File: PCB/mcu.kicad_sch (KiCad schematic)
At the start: 26 parts

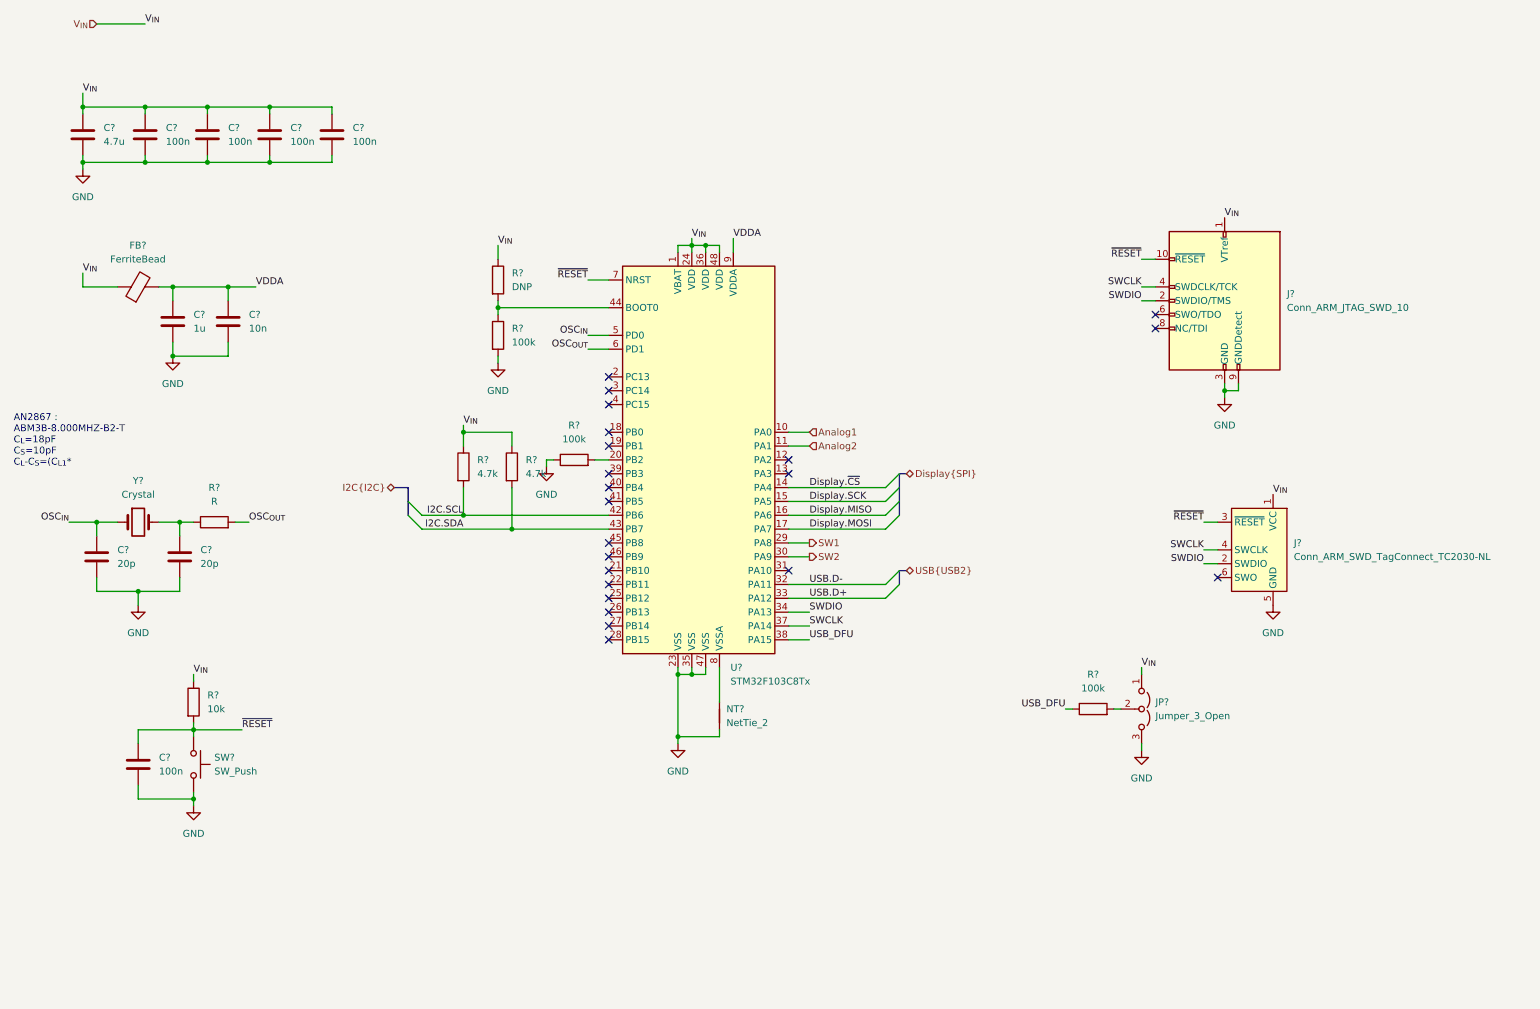
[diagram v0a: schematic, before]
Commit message: ok mcu
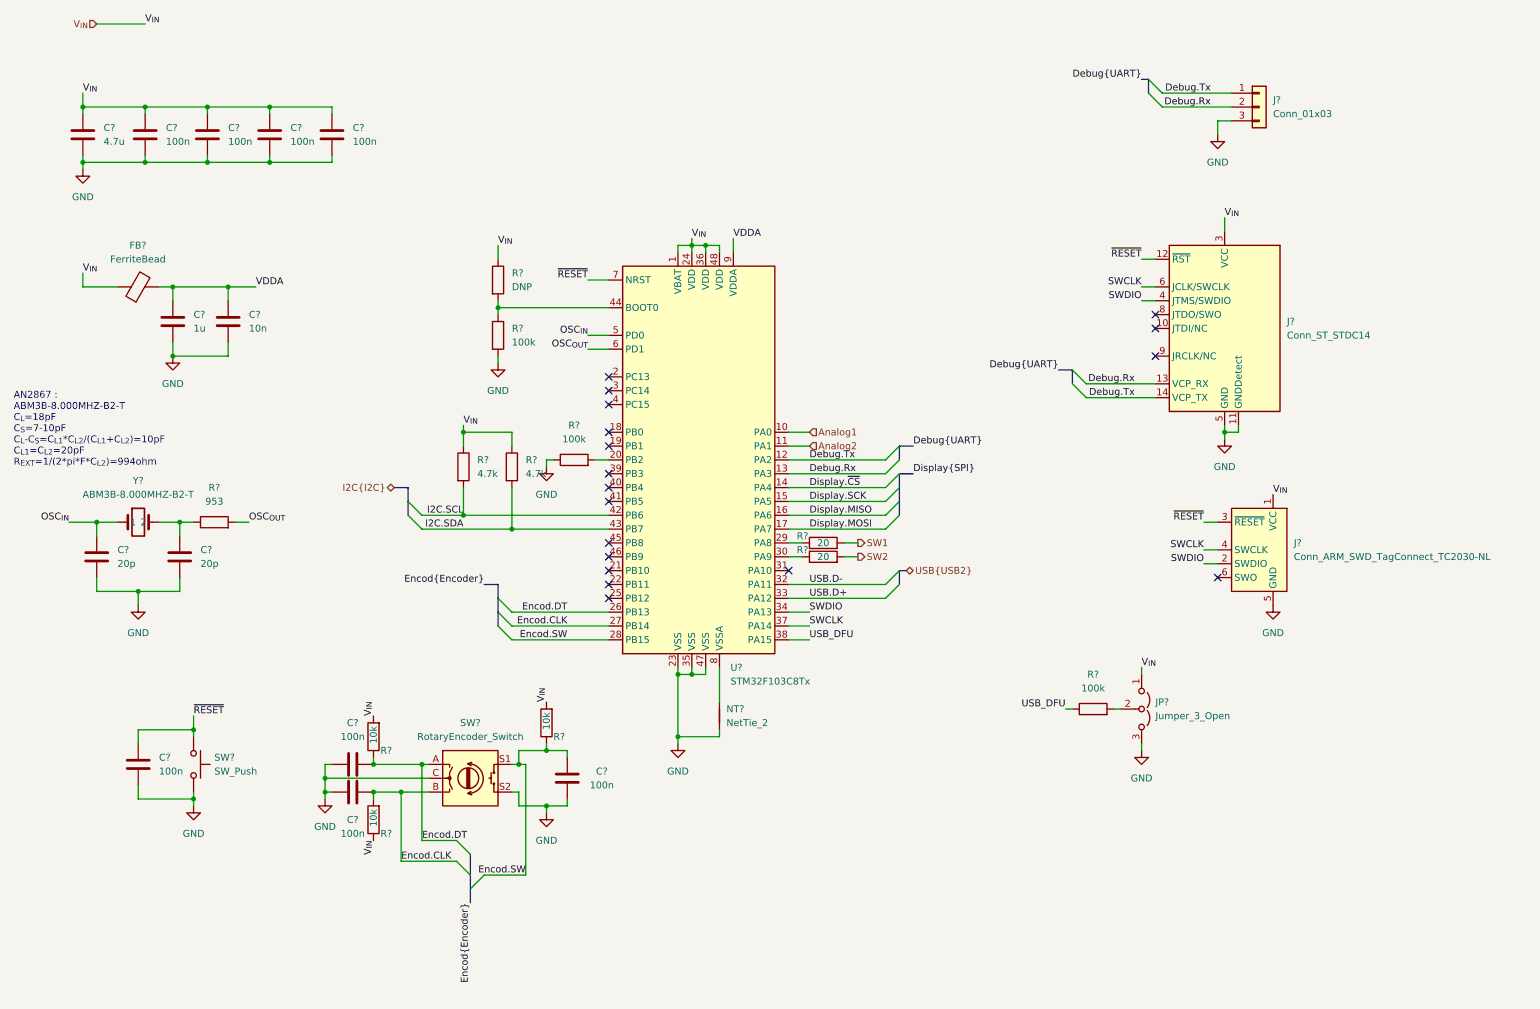
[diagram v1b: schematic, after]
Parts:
- removed J?: Conn_ARM_JTAG_SWD_10, symbol Connector:Conn_ARM_JTAG_SWD_10
- removed R?: 10k, symbol Device:R
- added C? (x3): 100n, symbol Device:C
- added J?: Conn_ST_STDC14, symbol Connector:Conn_ST_STDC14
- added J?: Conn_01x03, symbol Connector_Generic:Conn_01x03
- added R? (x3): 10k, symbol Device:R
- added R? (x2): 20, symbol Device:R
- added SW?: RotaryEncoder_Switch, symbol Device:RotaryEncoder_Switch
- R?: value R -> 953
- Y?: value Crystal -> ABM3B-8.000MHZ-B2-T; footprint (none) -> Crystal:Crystal_SMD_Abracon_ABM3B-4Pin_5.0x3.2mm
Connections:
- net GND: now also C?.1, C?.2, C?.2, J?.11 (GNDDetect), J?.3 (Pin_3), J?.5 (GND), J?.7 (GND), SW?.C, SW?.S2
- net SW1: now also R?.2; no longer U?.29 (PA8)
- net SW2: now also R?.2; no longer U?.30 (PA9)
- net SWCLK: now also J?.6 (JCLK/SWCLK)
- net SWDIO: now also J?.4 (JTMS/SWDIO)
- net V_{IN}: now also J?.3 (VCC), R?.1, R?.2, R?.2
- net ~{RESET}: now also J?.12 (~{RST})
- net Debug.Tx: now reaches U?.12 (PA2)
- net Debug.Tx: now also J?.1 (Pin_1), J?.14 (VCP_TX)
- net Debug.Rx: now reaches U?.13 (PA3)
- net Debug.Rx: now also J?.13 (VCP_RX), J?.2 (Pin_2)
- net Encod.DT: now reaches U?.26 (PB13)
- net Encod.DT: now also C?.2, R?.1, SW?.A
- net Encod.CLK: now reaches U?.27 (PB14)
- net Encod.CLK: now also C?.1, R?.2, SW?.B
- net Encod.SW: now reaches U?.28 (PB15)
- net Encod.SW: now also C?.1, R?.1, SW?.S1
- new net: R?.1, U?.29 (PA8)
- new net: R?.1, U?.30 (PA9)
- no-connect marks 22 -> 18
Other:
- note added: "AN2867 : ABM3B-8.000MHZ-B2-T C_{L}=18pF C_{S}=7-10pF C_{L}-C_{S}=C_{L1}*C_{L2}/(C_{L1}+C_{L2})=10pF C_{L1}=C_{L2}=20pF R_{EXT}=1/(2*pi*F*C_{L2})=994ohm"
- note removed: "AN2867 : ABM3B-8.000MHZ-B2-T C_{L}=18pF C_{S}=10pF C_{L}-C_{S}=(C_{L1}*"
